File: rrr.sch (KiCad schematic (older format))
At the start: 8 parts, among them J1 Conn_01x01_Male, J2 Conn_01x01_Male, J3 Conn_01x01_Male, J4 Conn_01x01_Male, J5 Conn_01x01_Male, J6 Conn_01x01_Male, K1 SILxx-1Axx-71x, K2 SILxx-1Axx-71x

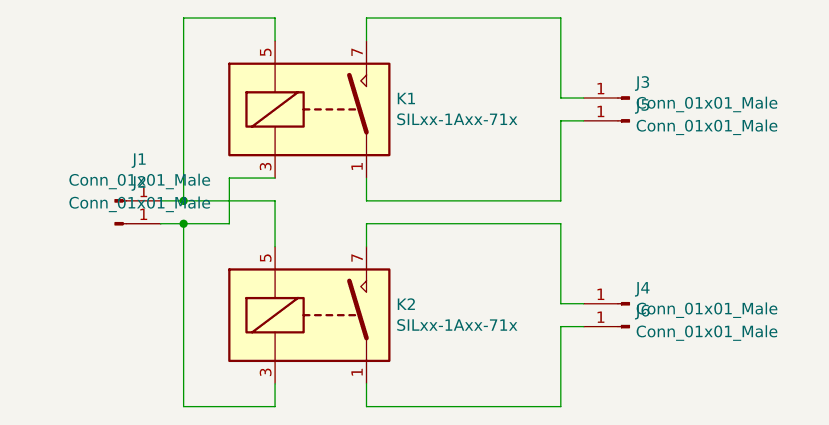
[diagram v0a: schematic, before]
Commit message: Initial commit for 25065637
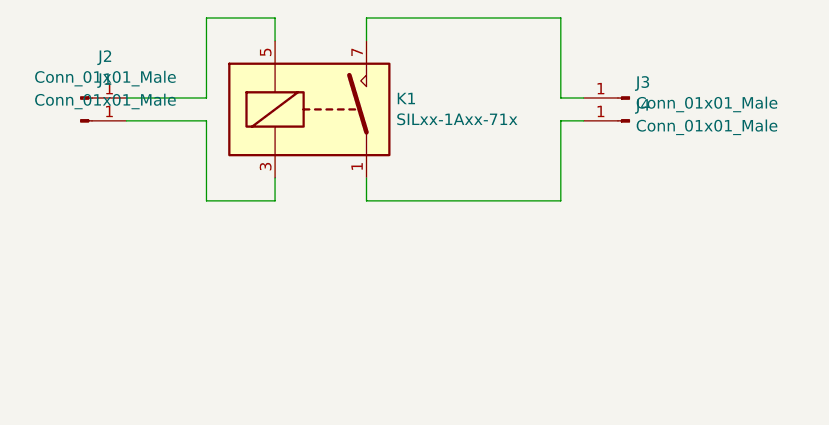
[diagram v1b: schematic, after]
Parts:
- removed J4, J6: Conn_01x01_Male, Connector_PinHeader_2.54mm:PinHeader_1x01_P2.54mm_Vertical, symbol Connector:Conn_01x01_Male
- removed K2: SILxx-1Axx-71x, Relay_THT:Relay_SPST_StandexMeder_SIL_Form1A, symbol Relay:SILxx-1Axx-71x
- renumbered J2 to J1, J1 to J2, J5 to J4
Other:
- moved on the sheet: J1, J2
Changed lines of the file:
@@
 	1    0    0    -1
 $EndComp
-$Comp
-L Relay:SILxx-1Axx-71x K2
-U 1 1 60EEBDC6
-P 5350 3700
-F 0 "K2" H 5680 3746 50  0000 L CNN
-F 1 "SILxx-1Axx-71x" H 5680 3655 50  0000 L CNN
-F 2 "Relay_THT:Relay_SPST_StandexMeder_SIL_Form1A" H 5700 3650 50  0001 L CNN
-F 3 "https://standexelectronics.com/wp-content/uploads/datasheet_reed_relay_SIL.pdf" H 5350 3700 50  0001 C CNN
-	1    5350 3700
-	1    0    0    -1
-$EndComp
-Wire Wire Line
-	4750 3200 4750 2400
-Wire Wire Line
-	4750 2400 5150 2400
-Wire Wire Line
-	5150 2400 5150 2500
-Wire Wire Line
-	4750 3300 4750 4100
-Wire Wire Line
-	4750 4100 5150 4100
-Wire Wire Line
-	5150 4100 5150 4000
-Wire Wire Line
-	5150 3100 4950 3100
-Wire Wire Line
-	4950 3100 4950 3300
-Wire Wire Line
-	4950 3300 4750 3300
-Wire Wire Line
-	4750 3200 5150 3200
-Wire Wire Line
-	5150 3200 5150 3400
-Wire Wire Line
-	6500 3650 6400 3650
-Wire Wire Line
-	6400 3650 6400 3300
-Wire Wire Line
-	6400 3300 5550 3300
-Wire Wire Line
-	5550 3300 5550 3400
-Wire Wire Line
-	6500 3750 6400 3750
-Wire Wire Line
-	6400 3750 6400 4100
-Wire Wire Line
-	6400 4100 5550 4100
-Wire Wire Line
-	5550 4100 5550 4000
 Wire Wire Line
 	5550 3100 5550 3200
@@
 	5550 2400 5550 2500
 $Comp
-L Connector:Conn_01x01_Male J1
+L Connector:Conn_01x01_Male J2
 U 1 1 60EF8135
-P 4450 3200
-F 0 "J1" H 4558 3381 50  0000 C CNN
-F 1 "Conn_01x01_Male" H 4558 3290 50  0000 C CNN
-F 2 "Connector_PinHeader_2.54mm:PinHeader_1x01_P2.54mm_Vertical" H 4450 3200 50  0001 C CNN
-F 3 "~" H 4450 3200 50  0001 C CNN
-	1    4450 3200
+P 4300 2750
+F 0 "J2" H 4408 2931 50  0000 C CNN
+F 1 "Conn_01x01_Male" H 4408 2840 50  0000 C CNN
+F 2 "Connector_PinHeader_2.54mm:PinHeader_1x01_P2.54mm_Vertical" H 4300 2750 50  0001 C CNN
+F 3 "~" H 4300 2750 50  0001 C CNN
+	1    4300 2750
 	1    0    0    -1
 $EndComp
 $Comp
-L Connector:Conn_01x01_Male J2
+L Connector:Conn_01x01_Male J1
 U 1 1 60EF87E2
-P 4450 3300
-F 0 "J2" H 4558 3481 50  0000 C CNN
-F 1 "Conn_01x01_Male" H 4558 3390 50  0000 C CNN
-F 2 "Connector_PinHeader_2.54mm:PinHeader_1x01_P2.54mm_Vertical" H 4450 3300 50  0001 C CNN
-F 3 "~" H 4450 3300 50  0001 C CNN
-	1    4450 3300
+P 4300 2850
+F 0 "J1" H 4408 3031 50  0000 C CNN
+F 1 "Conn_01x01_Male" H 4408 2940 50  0000 C CNN
+F 2 "Connector_PinHeader_2.54mm:PinHeader_1x01_P2.54mm_Vertical" H 4300 2850 50  0001 C CNN
+F 3 "~" H 4300 2850 50  0001 C CNN
+	1    4300 2850
 	1    0    0    -1
 $EndComp
@@
 $EndComp
 $Comp
-L Connector:Conn_01x01_Male J5
+L Connector:Conn_01x01_Male J4
 U 1 1 60EFA063
 P 6700 2850
-F 0 "J5" H 6672 2782 50  0000 R CNN
+F 0 "J4" H 6672 2782 50  0000 R CNN
 F 1 "Conn_01x01_Male" H 6672 2873 50  0000 R CNN
 F 2 "Connector_PinHeader_2.54mm:PinHeader_1x01_P2.54mm_Vertical" H 6700 2850 50  0001 C CNN
@@
 	-1   0    0    1
 $EndComp
-$Comp
-L Connector:Conn_01x01_Male J4
-U 1 1 60EFA770
-P 6700 3650
-F 0 "J4" H 6672 3582 50  0000 R CNN
-F 1 "Conn_01x01_Male" H 6672 3673 50  0000 R CNN
-F 2 "Connector_PinHeader_2.54mm:PinHeader_1x01_P2.54mm_Vertical" H 6700 3650 50  0001 C CNN
-F 3 "~" H 6700 3650 50  0001 C CNN
-	1    6700 3650
-	-1   0    0    1
-$EndComp
-$Comp
-L Connector:Conn_01x01_Male J6
-U 1 1 60EFAEB6
-P 6700 3750
-F 0 "J6" H 6672 3682 50  0000 R CNN
-F 1 "Conn_01x01_Male" H 6672 3773 50  0000 R CNN
-F 2 "Connector_PinHeader_2.54mm:PinHeader_1x01_P2.54mm_Vertical" H 6700 3750 50  0001 C CNN
-F 3 "~" H 6700 3750 50  0001 C CNN
-	1    6700 3750
-	-1   0    0    1
-$EndComp
 Wire Wire Line
-	4650 3200 4750 3200
-Connection ~ 4750 3200
+	4500 2750 4850 2750
 Wire Wire Line
-	4650 3300 4750 3300
-Connection ~ 4750 3300
+	4850 2750 4850 2400
+Wire Wire Line
+	4850 2400 5150 2400
+Wire Wire Line
+	5150 2400 5150 2500
+Wire Wire Line
+	4500 2850 4850 2850
+Wire Wire Line
+	4850 2850 4850 3200
+Wire Wire Line
+	4850 3200 5150 3200
+Wire Wire Line
+	5150 3200 5150 3100
 $EndSCHEMATC
